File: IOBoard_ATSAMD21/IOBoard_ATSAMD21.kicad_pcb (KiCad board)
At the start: 2 copper layers, 76.2 x 128.5 mm, 36 parts, among them J1 Conn_PIC_ICSP_ICD, J2 Conn_01x04_Male, SW1 EG_1218, SW2 EG_1218, SW3 EG_1218, SW4 EG_1218, U1 ATSAMD21G18A-A, U2 AP2112K-3.3

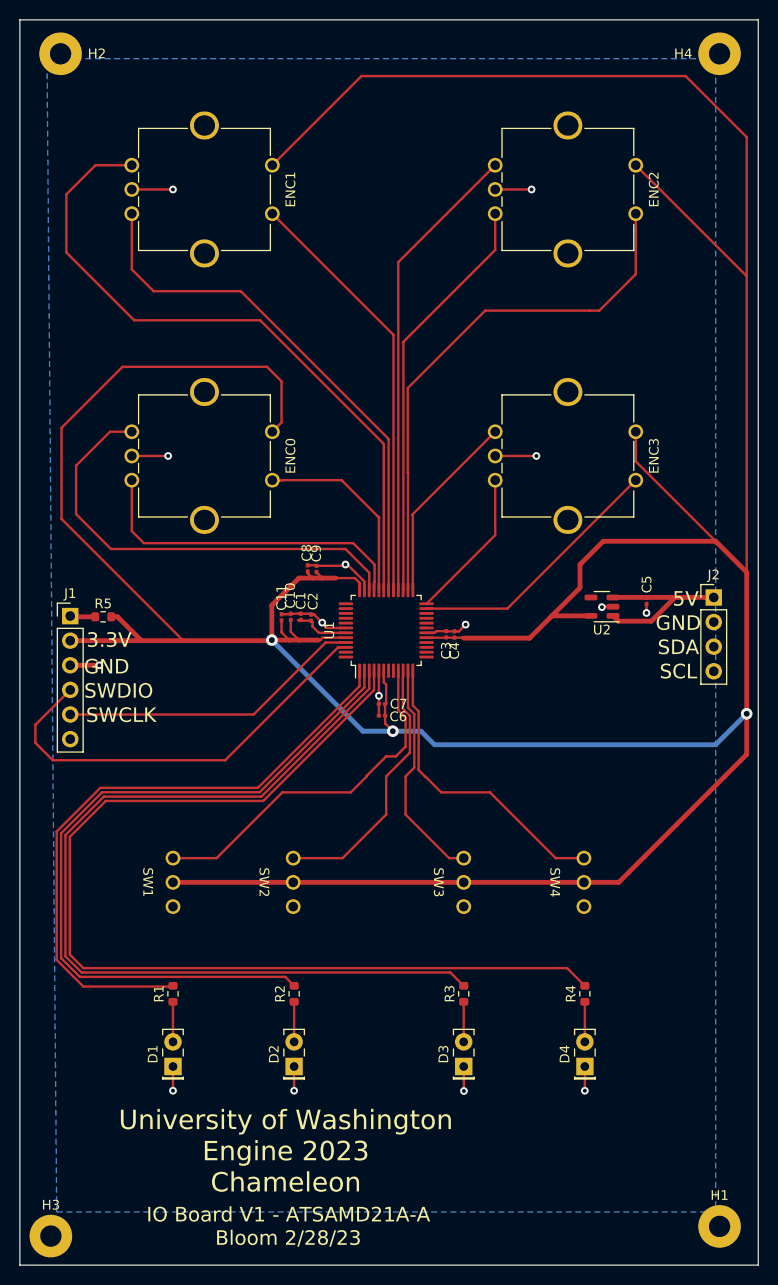
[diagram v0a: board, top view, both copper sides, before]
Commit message: updating lab PC
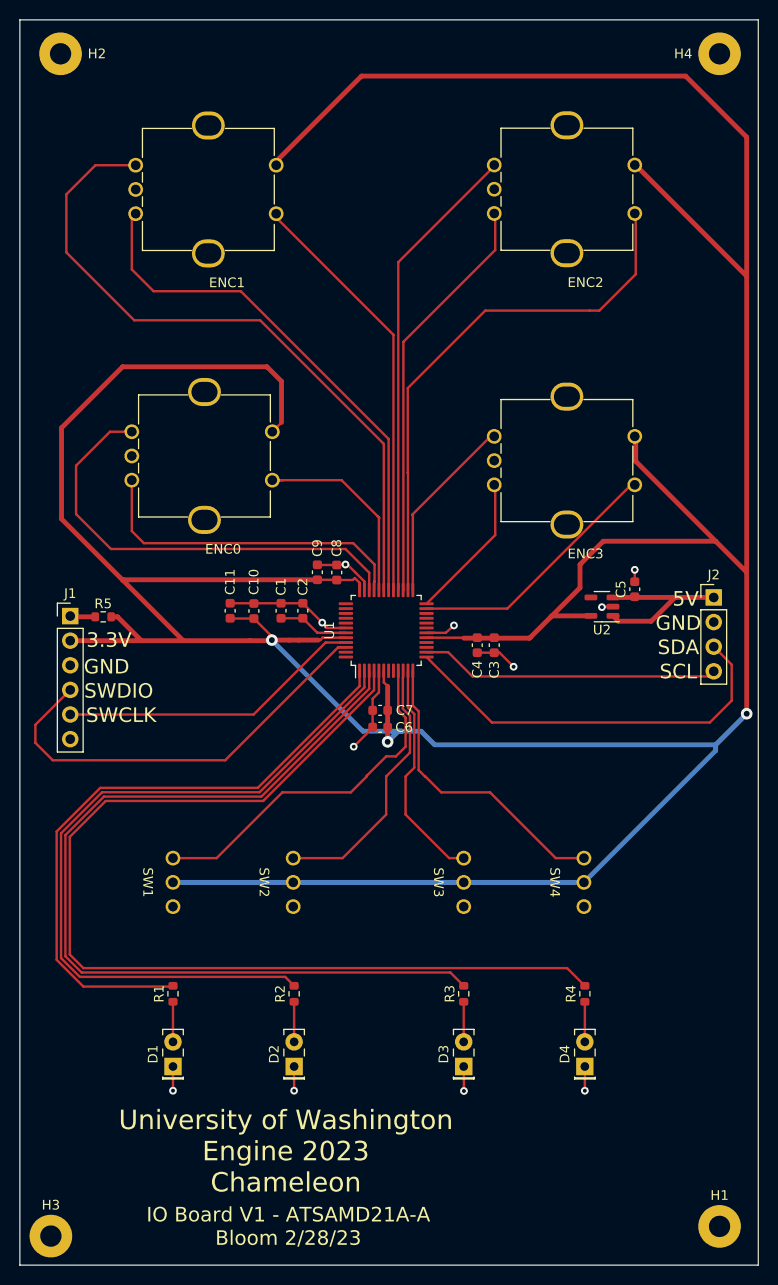
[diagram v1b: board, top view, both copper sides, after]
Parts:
- C1, C10, C11, C2, C3, C4, C5, C6, C7, C8, C9: footprint Capacitor_SMD:C_0201_0603Metric -> Capacitor_SMD:C_0603_1608Metric
- ENC0, ENC1, ENC2, ENC3: footprint Rotary_Encoder:RotaryEncoder_Bourns_Vertical_PEC12R-3xxxF-Sxxxx -> custom_lib:PEC12R-3217F-S0024-ND
- moved ENC3 16.1 mm to (124.2, 97.1)
- moved ENC1 16.0 mm to (87.2, 69.1)
- moved ENC0 15.7 mm to (86.8, 96.6)
- moved ENC2 15.7 mm to (124.2, 69.1)
- moved C11 5.34 mm to (87.5, 102.5)
- moved C3 5.08 mm to (114.8, 106.0), turned to -90 degrees
- moved C10 3.85 mm to (90.0, 102.5)
- moved C8 3.03 mm to (98.5, 98.5)
- moved C4 2.60 mm to (113.0, 106.0), turned to 90 degrees
- moved C1 2.14 mm to (92.8, 102.5)
- moved C5 1.71 mm to (129.2, 100.2), turned to 90 degrees
- moved C6 1.22 mm to (103.0, 114.5)
- moved C2 1.10 mm to (95.0, 102.5)
- moved C7 0.68 mm to (103.0, 112.8)
- moved C9 0.36 mm to (96.5, 98.5)
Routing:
- net /SDA: track 0.00 -> 41.6 mm
- net /SCL: track 0.00 -> 30.9 mm
- net GND: track 55.3 -> 48.6 mm, vias 15 -> 11
- net +3.3V: track 433.0 -> 438.6 mm
- net Net-(C1-Pad2): track 5.75 -> 7.31 mm
- removed copper zone on B.Cu, net GND
